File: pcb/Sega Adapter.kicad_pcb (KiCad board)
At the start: 2 copper layers, 6 parts, among them J1 Sega, J2 Atari, J3 ICSP, SW1 C64, U1 PIC16F1847

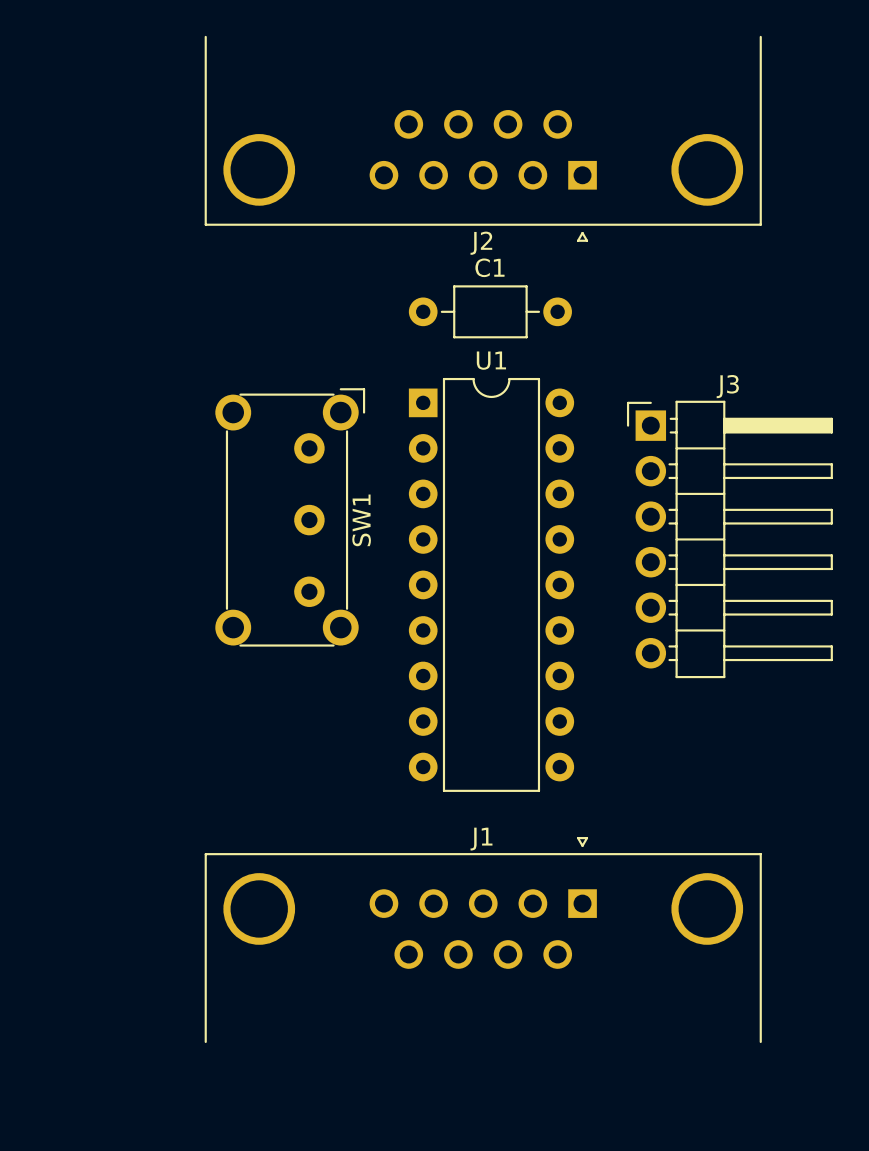
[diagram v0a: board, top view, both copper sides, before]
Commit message: Finished schematic
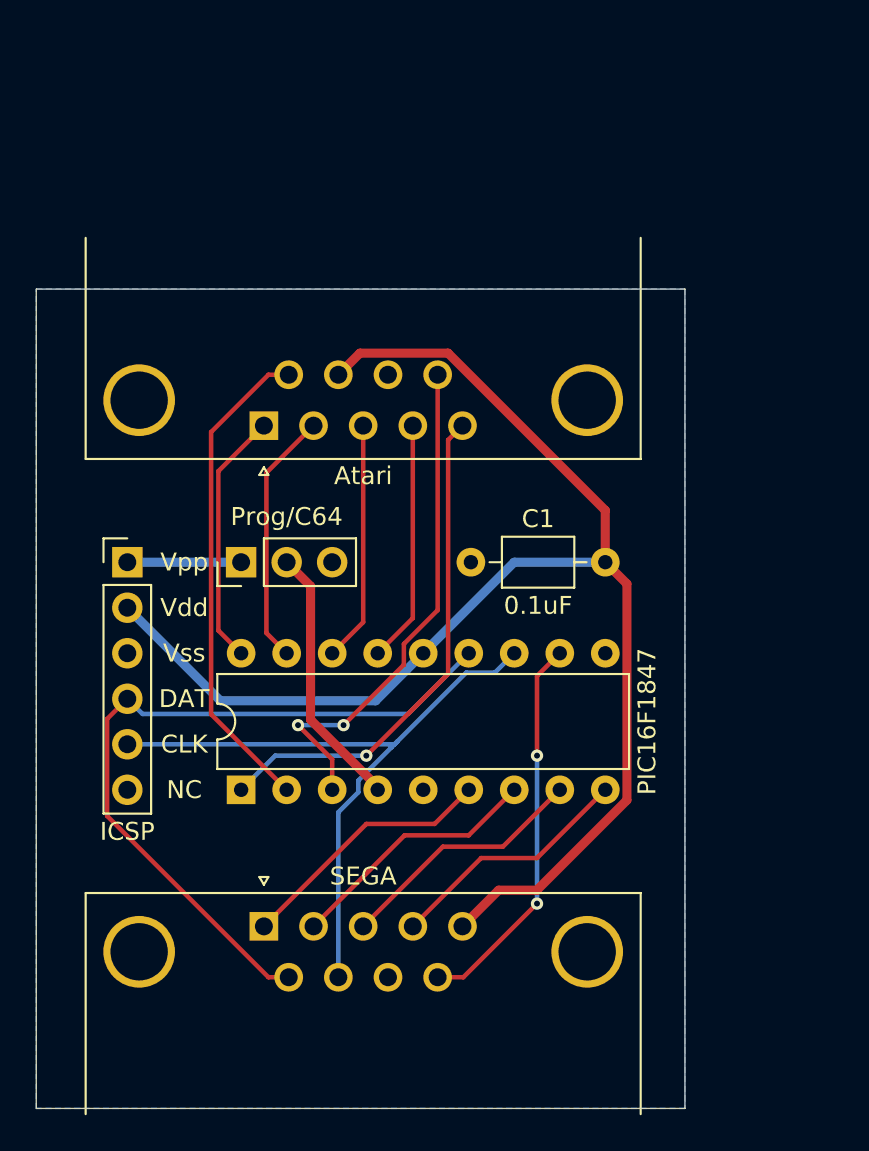
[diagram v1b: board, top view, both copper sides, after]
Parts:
- removed SW1: C64, Button_Switch_THT:SW_E-Switch_EG1224_SPDT_Angled
- added JP1: Prog/C64, Connector_PinHeader_2.54mm:PinHeader_1x03_P2.54mm_Vertical, F.Cu at (139.7, 115.6)
- Atari: renamed from J2; footprint Connector_Dsub:DSUB-9_Male_Horizontal_P2.77x2.84mm_EdgePinOffset4.94mm_Housed_MountingHolesOffset7.48mm -> Connector_Dsub:DSUB-9_Female_Horizontal_P2.77x2.84mm_EdgePinOffset7.70mm_Housed_MountingHolesOffset9.12mm
- J3: footprint Connector_PinHeader_2.54mm:PinHeader_1x06_P2.54mm_Horizontal -> Connector_PinHeader_2.54mm:PinHeader_1x06_P2.54mm_Vertical
- SEGA: renamed from J1; footprint Connector_Dsub:DSUB-9_Female_Horizontal_P2.77x2.84mm_EdgePinOffset4.94mm_Housed_MountingHolesOffset7.48mm -> Connector_Dsub:DSUB-9_Male_Horizontal_P2.77x2.84mm_EdgePinOffset7.70mm_Housed_MountingHolesOffset9.12mm
- moved J3 30.2 mm to (133.3, 115.6)
- moved U1 23.9 mm to (139.7, 128.3), turned to 90 degrees
- moved Atari 22.6 mm to (141.0, 108.0)
- moved SEGA 17.8 mm to (141.0, 135.9)
- moved C1 14.2 mm to (152.5, 115.6)
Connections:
- net Net-(C1-Pad2) renamed +5V
- Atari pad 0: Net-(J2-Pad0) -> GND
- Atari pad 8: Net-(C1-Pad1) -> GND
- C1 pad 1: Net-(C1-Pad1) -> GND
- J3 pad 3: Net-(C1-Pad1) -> GND
- SEGA pad 0: Net-(J1-Pad0) -> GND
- SEGA pad 8: Net-(C1-Pad1) -> GND
- U1 pad 5: Net-(C1-Pad1) -> GND
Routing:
- net +5V: track 0.00 -> 79.8 mm
- net Net-(J1-Pad6): track 0.00 -> 41.7 mm
- net Net-(J1-Pad7): track 0.00 -> 38.4 mm
- net Net-(J2-Pad9): track 0.00 -> 28.8 mm, vias 0 -> 2
- net Net-(J2-Pad5): track 0.00 -> 28.4 mm, vias 0 -> 1
- net Net-(J2-Pad6): track 0.00 -> 27.4 mm
- net Net-(J1-Pad9): track 0.00 -> 21.7 mm, vias 0 -> 2
- net Net-(JP1-Pad2): track 0.00 -> 14.8 mm
- net Net-(J1-Pad1): track 0.00 -> 14.6 mm
- net Net-(J1-Pad2): track 0.00 -> 14.4 mm
- net Net-(J2-Pad1): track 0.00 -> 14.3 mm
- net Net-(J2-Pad2): track 0.00 -> 14.3 mm
- net Net-(J1-Pad3): track 0.00 -> 14.1 mm
- net Net-(J1-Pad4): track 0.00 -> 13.9 mm
- net Net-(J2-Pad4): track 0.00 -> 13.5 mm
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- added copper zone on B.Cu, net GND
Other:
- board outline added: 36.2 x 45.7 mm
- net class Default: clearance 0.2 -> 0.1524; trace_width 0.25 -> 0.1524; via_dia 0.8 -> 0.6858; via_drill 0.4 -> 0.3302
- rule pad_to_mask_clearance: 0 -> 0.0508
- rule trace_clearance: 0.2 -> 0.1524
- rule trace_min: 0.2 -> 0.1524
- rule via_min_drill: 0.3 -> 0.254
- rule via_min_size: 0.4 -> 0.508
- board text added: "CLK"
- board text added: "DAT"
- board text added: "NC"
- board text added: "Vdd"
- board text added: "Vpp"
- board text added: "Vss"
